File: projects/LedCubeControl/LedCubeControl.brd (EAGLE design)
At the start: 30.1 x 69.8 mm, 29 parts, among them IC1 74HC595N, IC2 74HC595N, IC3 74HC595N, T1 PN2222A, T2 PN2222A, T3 PN2222A, T4 PN2222A

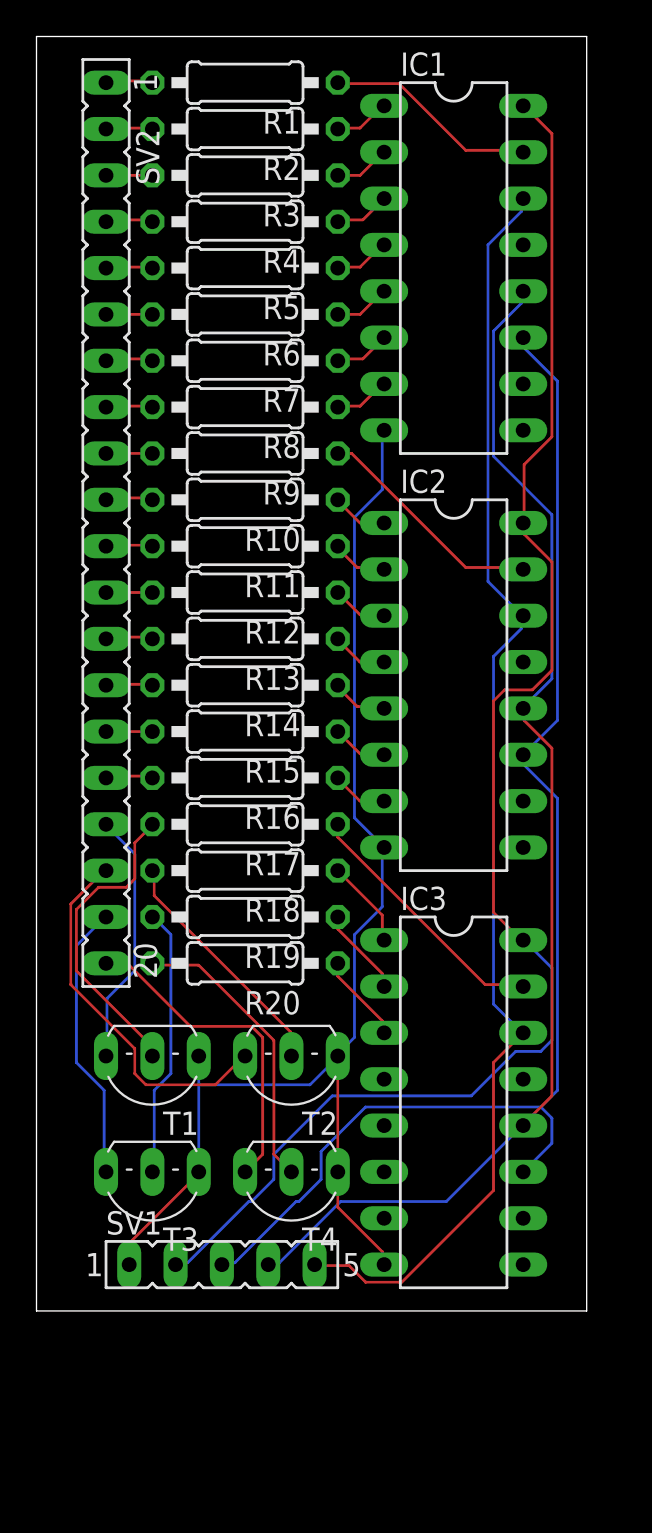
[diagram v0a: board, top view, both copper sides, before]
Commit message: fix: small fixes applied
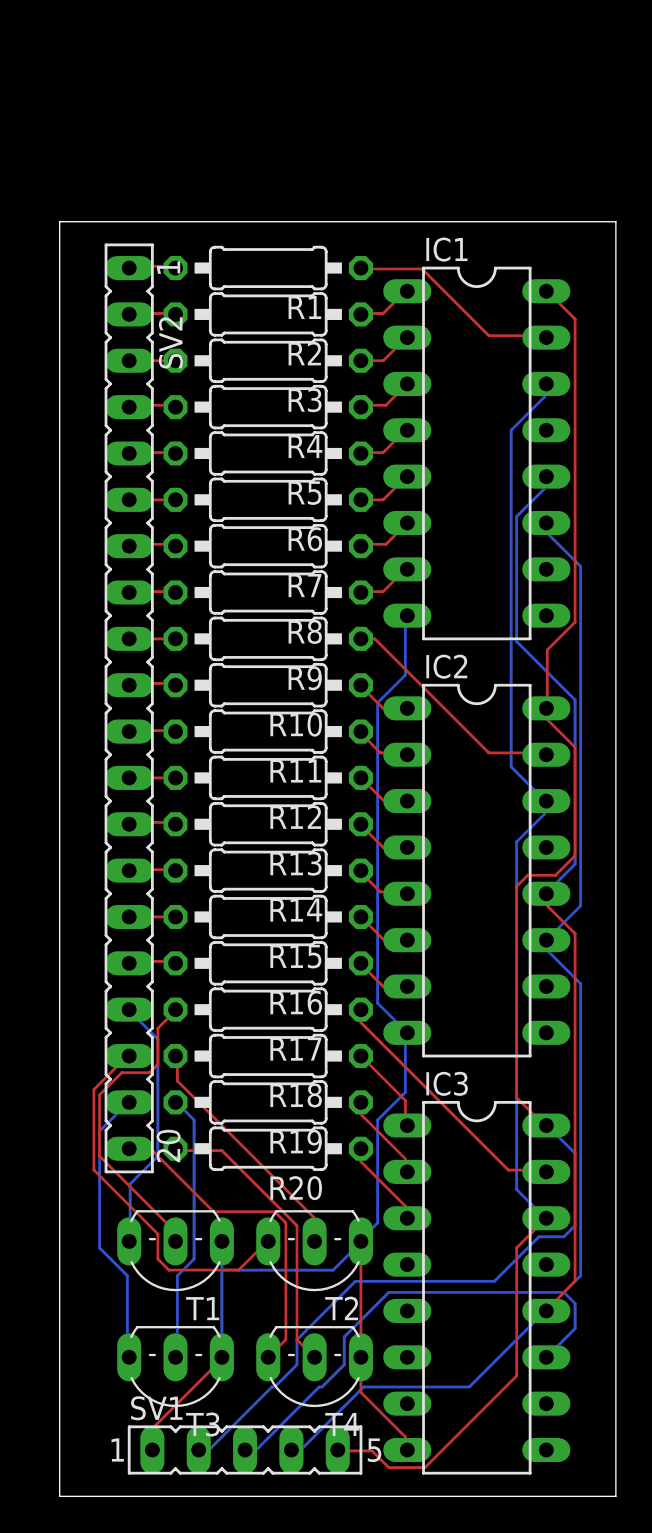
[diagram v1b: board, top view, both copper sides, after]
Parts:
- moved R2 10.2 mm to (11.4, 64.8)
- moved IC1 10.2 mm to (22.9, 57.1)
- moved IC2 10.2 mm to (22.9, 34.3)
- moved R11 10.2 mm to (11.4, 41.9)
- moved R12 10.2 mm to (11.4, 39.4)
- moved R13 10.2 mm to (11.4, 36.8)
- moved R14 10.2 mm to (11.4, 34.3)
- moved R3 10.2 mm to (11.4, 62.2)
- moved R5 10.2 mm to (11.4, 57.1)
- moved SV2 10.2 mm to (3.81, 43.2)
- moved T3 10.2 mm to (6.35, 6.35)
- moved T4 10.2 mm to (14.0, 6.35)
- moved IC3 10.2 mm to (22.9, 11.4)
- moved R18 10.2 mm to (11.4, 24.1)
- moved R19 10.2 mm to (11.4, 21.6)
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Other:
- board size 30.1 x 69.8 mm -> 30.5 x 69.8 mm
